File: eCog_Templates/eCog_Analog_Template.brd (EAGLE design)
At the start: 48 x 28 mm, 10 parts

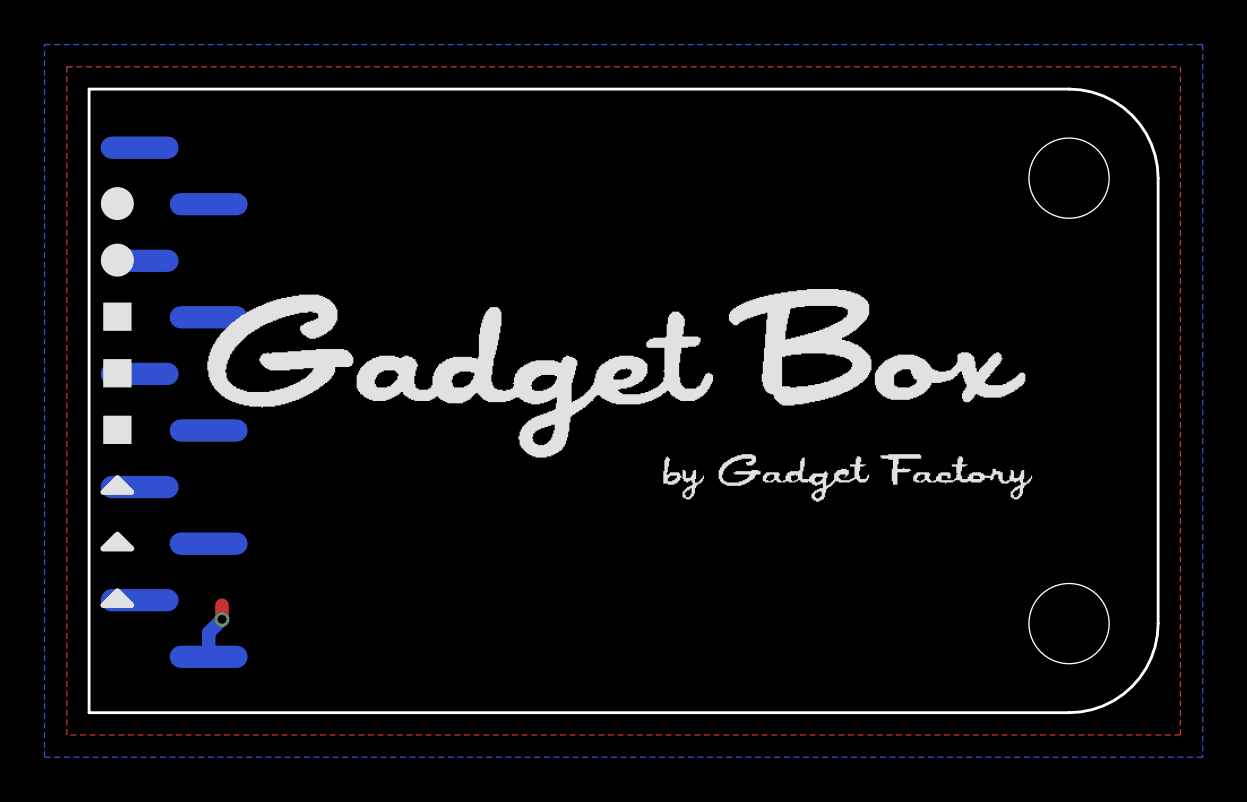
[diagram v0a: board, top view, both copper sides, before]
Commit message: All the 2.0 updates
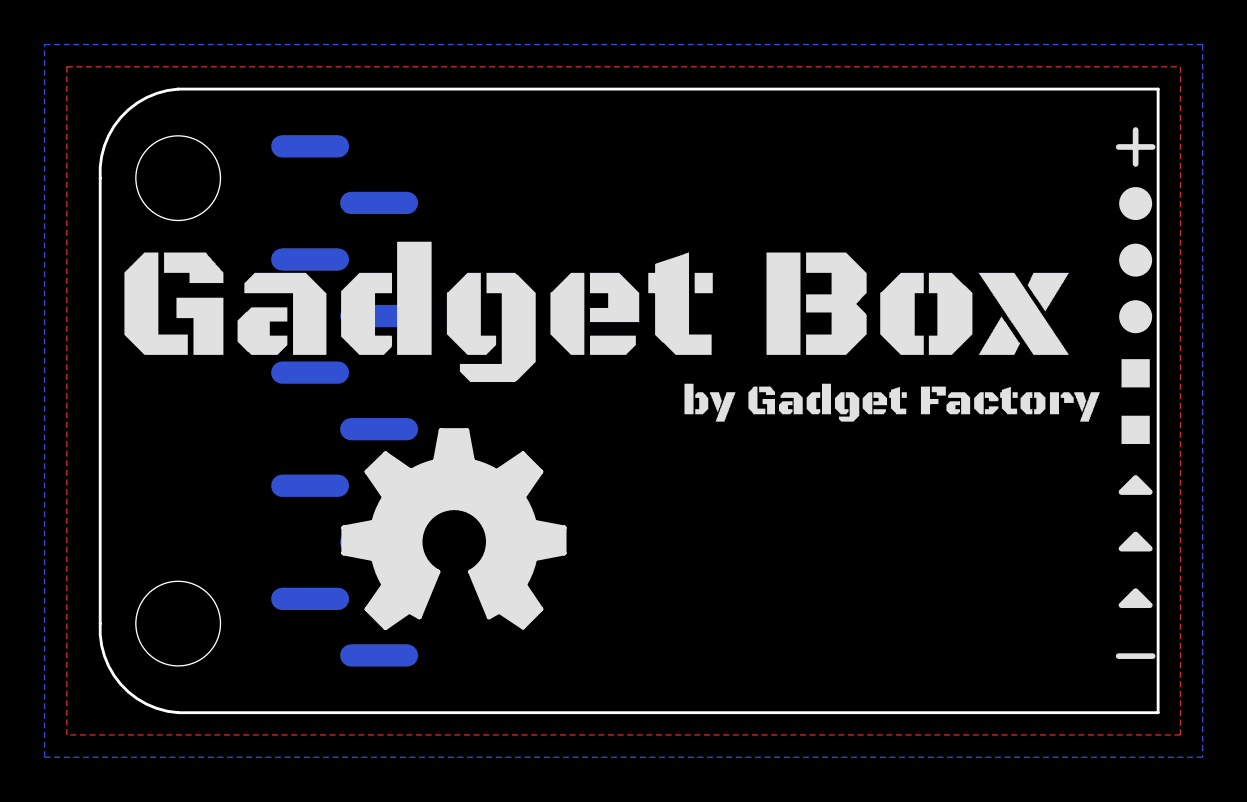
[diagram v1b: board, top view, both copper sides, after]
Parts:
- added U$10: (no value), ohw-logo:OSHW_FILLX350_NOTEXT
- U$1: device GadgetFactory:GADGETBOX_TEXT -> eCogs:LEGEND_DIO
- U$4: device eCogs:LEGEND_PWM -> GadgetFactory:GADGETBOX_TEXT
- moved U$2 45.7 mm to (47.0, 22.9)
- moved U$3 45.7 mm to (47.0, 20.3)
- moved U$5 45.7 mm to (47.0, 15.2)
- moved U$6 45.7 mm to (47.0, 12.7)
- moved U$7 45.7 mm to (47.0, 10.2)
- moved U$8 45.7 mm to (47.0, 7.62)
- moved U$9 45.7 mm to (47.0, 5.08)
- moved U$1 23.0 mm to (47.0, 17.8)
- moved U$4 21.6 mm to (22.9, 17.8)
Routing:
- net 3V3: track 2.56 -> 0.00 mm, vias 1 -> 0
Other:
- board size 48 x 28 mm -> 47.5 x 28 mm
- board text added: "ecog100 v2.0"
- board text removed: "ecog100 v1.0"
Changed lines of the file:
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@@
 <plain>
 <text x="37.559" y="18.415" size="0.8128" layer="22" font="vector" rot="MR0">ecog100.GadgetFactory.net</text>
-<text x="39.702" y="2.159" size="1.016" layer="22" font="vector" rot="MR0">ecog100 v1.0</text>
+<text x="39.702" y="2.159" size="1.016" layer="22" font="vector" rot="MR0">ecog100 v2.0</text>
 <text x="39.702" y="3.429" size="1.016" layer="22" font="vector" rot="MR0">Project Name</text>
 <text x="39.702" y="4.699" size="1.016" layer="22" font="vector" rot="MR0">eCogs</text>
-<text x="11.335" y="19.812" size="1.016" layer="22" font="vector" rot="MR0">G1&lt;&gt;</text>
-<text x="11.335" y="17.272" size="1.016" layer="22" font="vector" rot="MR0">G2&lt;&gt;</text>
-<text x="11.335" y="14.732" size="1.016" layer="22" font="vector" rot="MR0">G3&lt;&gt;</text>
-<text x="11.335" y="12.192" size="1.016" layer="22" font="vector" rot="MR0">G4&lt;&gt;</text>
-<text x="11.335" y="9.652" size="1.016" layer="22" font="vector" rot="MR0">G5&lt;&gt;</text>
-<text x="11.335" y="7.112" size="1.016" layer="22" font="vector" rot="MR0">G6&lt;&gt;</text>
-<text x="11.335" y="4.572" size="1.016" layer="22" font="vector" rot="MR0">G7&lt;&gt;</text>
-<text x="11.335" y="22.352" size="1.016" layer="22" font="vector" rot="MR0">G0&lt;&gt;</text>
+<text x="16.605" y="8.128" size="1.016" layer="22" font="vector" rot="MR180">G1&lt;&gt;</text>
+<text x="16.605" y="10.668" size="1.016" layer="22" font="vector" rot="MR180">G2&lt;&gt;</text>
+<text x="16.605" y="13.208" size="1.016" layer="22" font="vector" rot="MR180">G3&lt;&gt;</text>
+<text x="16.605" y="15.748" size="1.016" layer="22" font="vector" rot="MR180">G4&lt;&gt;</text>
+<text x="16.605" y="18.288" size="1.016" layer="22" font="vector" rot="MR180">G5&lt;&gt;</text>
+<text x="16.605" y="20.828" size="1.016" layer="22" font="vector" rot="MR180">G6&lt;&gt;</text>
+<text x="16.605" y="23.368" size="1.016" layer="22" font="vector" rot="MR180">G7&lt;&gt;</text>
+<text x="16.605" y="5.588" size="1.016" layer="22" font="vector" rot="MR180">G0&lt;&gt;</text>
 <text x="33.782" y="17.526" size="0.6096" layer="22" font="vector" rot="MR0">Copyright 2016</text>
 <text x="35.512" y="16.637" size="0.6096" layer="22" font="vector" rot="MR0">Gadget Factory, LLC</text>
-<text x="11.335" y="2.032" size="1.016" layer="22" font="vector" rot="MR0">3.3V</text>
-<text x="11.335" y="24.892" size="1.016" layer="22" font="vector" rot="MR0">GND</text>
+<text x="16.605" y="25.908" size="1.016" layer="22" font="vector" rot="MR180">3.3V</text>
+<text x="16.605" y="3.048" size="1.016" layer="22" font="vector" rot="MR180">GND</text>
+<wire x1="46.99" y1="26.162" x2="46.99" y2="24.638" width="0.254" layer="21"/>
+<wire x1="46.228" y1="25.4" x2="47.752" y2="25.4" width="0.254" layer="21"/>
+<wire x1="46.228" y1="2.54" x2="47.752" y2="2.54" width="0.254" layer="21"/>
 </plain>
 <attributes>
@@
 </autorouter>
 <elements>
-<element name="ECOG" library="eCogs" package="ECOG_GENERAL_SMD" value="ECOG_GENERAL_ROWECOG_GENERAL_SMD" x="0" y="0" smashed="yes"/>
-<element name="U$1" library="GadgetFactory" package="GADGETBOX_TEXT" value="" x="24.13" y="15.24"/>
-<element name="U$2" library="eCogs" package="LEGEND_DIO" value="" x="1.27" y="22.86"/>
-<element name="U$3" library="eCogs" package="LEGEND_DIO" value="" x="1.27" y="20.32"/>
-<element name="U$4" library="eCogs" package="LEGEND_PWM" value="" x="1.27" y="17.78"/>
-<element name="U$5" library="eCogs" package="LEGEND_PWM" value="" x="1.27" y="15.24"/>
-<element name="U$6" library="eCogs" package="LEGEND_PWM" value="" x="1.27" y="12.7"/>
-<element name="U$7" library="eCogs" package="LEGEND_ANALOG" value="" x="1.27" y="10.16"/>
-<element name="U$8" library="eCogs" package="LEGEND_ANALOG" value="" x="1.27" y="7.62"/>
-<element name="U$9" library="eCogs" package="LEGEND_ANALOG" value="" x="1.27" y="5.08"/>
+<element name="ECOG" library="eCogs" package="ECOG_GENERAL_SMD" value="ECOG_GENERAL_ROWECOG_GENERAL_SMD" x="0" y="0" smashed="yes">
+<attribute name="DIGIKEY" value="S1013EC-10-ND" x="0" y="0" size="1.778" layer="27" display="off"/>
+</element>
+<element name="U$2" library="eCogs" package="LEGEND_DIO" value="" x="46.99" y="22.86"/>
+<element name="U$3" library="eCogs" package="LEGEND_DIO" value="" x="46.99" y="20.32"/>
+<element name="U$5" library="eCogs" package="LEGEND_PWM" value="" x="46.99" y="15.24"/>
+<element name="U$6" library="eCogs" package="LEGEND_PWM" value="" x="46.99" y="12.7"/>
+<element name="U$7" library="eCogs" package="LEGEND_ANALOG" value="" x="46.99" y="10.16"/>
+<element name="U$8" library="eCogs" package="LEGEND_ANALOG" value="" x="46.99" y="7.62"/>
+<element name="U$9" library="eCogs" package="LEGEND_ANALOG" value="" x="46.99" y="5.08"/>
+<element name="U$1" library="eCogs" package="LEGEND_DIO" value="" x="46.99" y="17.78"/>
+<element name="U$4" library="GadgetFactory" package="GADGETBOX_TEXT" value="" x="22.86" y="17.78"/>
+<element name="U$10" library="ohw-logo" package="OSHW_FILLX350_NOTEXT" value="" x="11.43" y="3.81"/>
 </elements>
 <signals>
@@
 <vertex x="-1" y="-1"/>
 </polygon>
-<wire x1="5.3694" y1="2.51" x2="5.3694" y2="3.5914" width="0.6096" layer="16"/>
-<wire x1="5.3694" y1="3.5914" x2="5.969" y2="4.191" width="0.6096" layer="16"/>
-<via x="5.969" y="4.191" extent="1-16" drill="0.381"/>
-<wire x1="5.969" y1="4.191" x2="5.969" y2="4.826" width="0.6096" layer="1"/>
 </signal>
 <signal name="A1">
